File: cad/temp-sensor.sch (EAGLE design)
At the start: 68 parts, among them Q1 300S14-U, Q2 320S14-U, Q3 320S14-U, U1 SE555D, U2 SE555D, U4 MCP6001UT-I/OT, U5 MCP6001UT-I/OT, U6 MCP6001UT-I/OT, U7 MCP6001UT-I/OT, U8 NCV4264-2CST50T3G, U9 ATMEGA328P_TQFP, Y1 16MHz

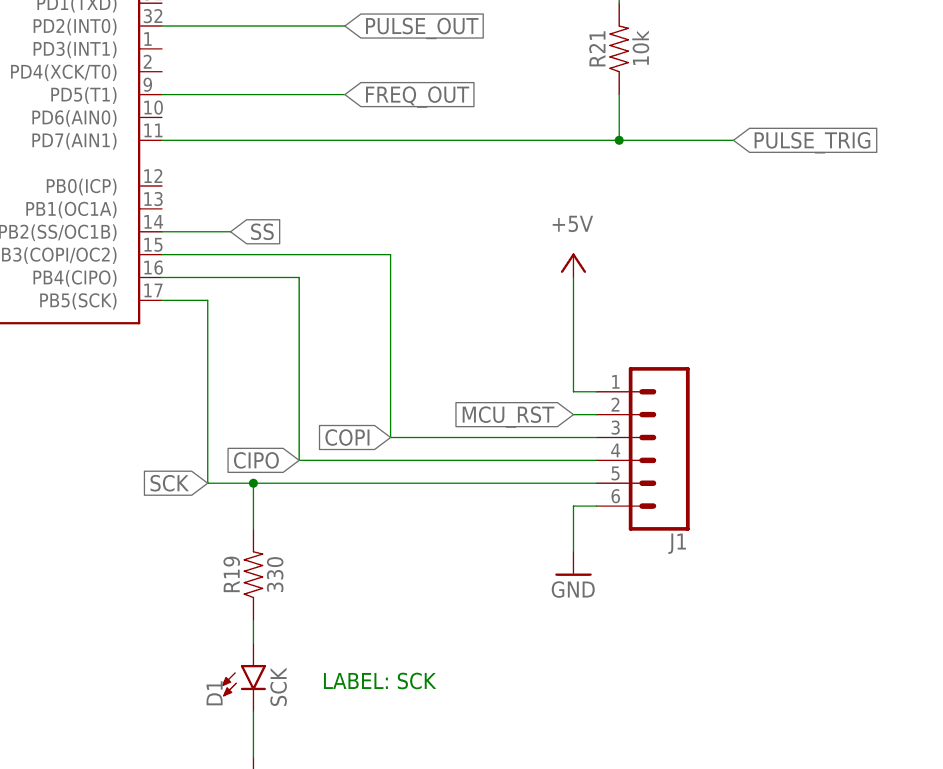
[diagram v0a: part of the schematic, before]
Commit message: Finishing touches on silk
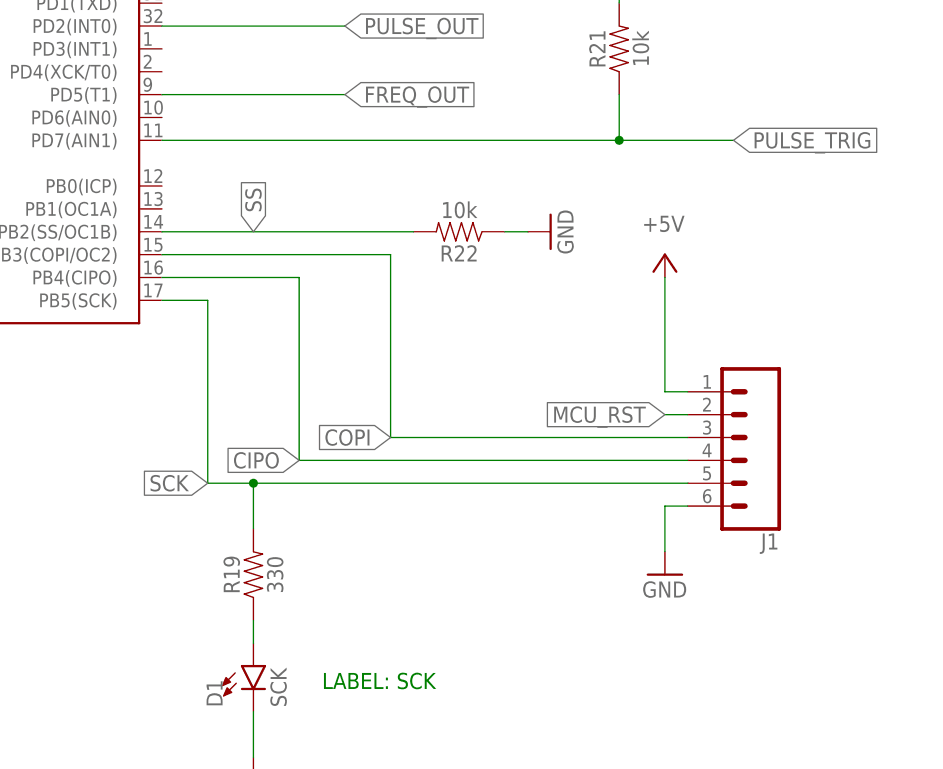
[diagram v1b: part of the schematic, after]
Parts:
- added R22: 10k, SparkFun-Resistors:10KOHM-0603-1/10W-1%
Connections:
- net GND: now also R22.1
- net SS: now also R22.2
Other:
- moved on the sheet: J1
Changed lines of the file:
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@@
 <part name="J2" library="SparkFun-Connectors" library_urn="urn:adsk.eagle:library:513" deviceset="CONN_04" device="PTH" package3d_urn="urn:adsk.eagle:package:38085/2"/>
 <part name="P+22" library="supply1" library_urn="urn:adsk.eagle:library:371" deviceset="+5V" device=""/>
+<part name="R22" library="SparkFun-Resistors" library_urn="urn:adsk.eagle:library:532" deviceset="10KOHM" device="-0603-1/10W-1%" package3d_urn="urn:adsk.eagle:package:41389018/1" value="10k"/>
+<part name="GND49" library="supply1" library_urn="urn:adsk.eagle:library:371" deviceset="GND" device=""/>
 </parts>
 <sheets>
@@
 <attribute name="VALUE" x="-177.038" y="226.06" size="1.778" layer="96" font="vector" rot="R270" align="top-center"/>
 </instance>
-<instance part="J1" gate="J1" x="-63.5" y="60.96" smashed="yes" rot="R180">
-<attribute name="VALUE" x="-58.42" y="70.866" size="1.778" layer="96" font="vector" rot="R180"/>
-<attribute name="NAME" x="-58.42" y="50.292" size="1.778" layer="95" font="vector" rot="R180"/>
-</instance>
-<instance part="GND39" gate="1" x="-71.12" y="45.72" smashed="yes">
-<attribute name="VALUE" x="-73.66" y="43.18" size="1.778" layer="96"/>
-</instance>
-<instance part="P+17" gate="1" x="-71.12" y="81.28" smashed="yes">
-<attribute name="VALUE" x="-73.66" y="83.82" size="1.778" layer="96"/>
+<instance part="J1" gate="J1" x="-53.34" y="60.96" smashed="yes" rot="R180">
+<attribute name="VALUE" x="-48.26" y="70.866" size="1.778" layer="96" font="vector" rot="R180"/>
+<attribute name="NAME" x="-48.26" y="50.292" size="1.778" layer="95" font="vector" rot="R180"/>
+</instance>
+<instance part="GND39" gate="1" x="-60.96" y="45.72" smashed="yes">
+<attribute name="VALUE" x="-63.5" y="43.18" size="1.778" layer="96"/>
+</instance>
+<instance part="P+17" gate="1" x="-60.96" y="81.28" smashed="yes">
+<attribute name="VALUE" x="-63.5" y="83.82" size="1.778" layer="96"/>
 </instance>
 <instance part="P+18" gate="1" x="-195.58" y="147.32" smashed="yes">
@@
 <instance part="P+22" gate="1" x="-38.1" y="137.16" smashed="yes">
 <attribute name="VALUE" x="-40.64" y="139.7" size="1.778" layer="96"/>
+</instance>
+<instance part="R22" gate="G$1" x="-83.82" y="83.82" smashed="yes" rot="R180">
+<attribute name="NAME" x="-83.82" y="82.296" size="1.778" layer="95" font="vector" rot="R180" align="bottom-center"/>
+<attribute name="VALUE" x="-83.82" y="85.344" size="1.778" layer="96" font="vector" rot="R180" align="top-center"/>
+</instance>
+<instance part="GND49" gate="1" x="-73.66" y="83.82" smashed="yes" rot="R90">
+<attribute name="VALUE" x="-71.12" y="81.28" size="1.778" layer="96" rot="R90"/>
 </instance>
 </instances>
@@
 <segment>
 <pinref part="J1" gate="J1" pin="6"/>
-<wire x1="-68.58" y1="53.34" x2="-71.12" y2="53.34" width="0.1524" layer="91"/>
-<wire x1="-71.12" y1="53.34" x2="-71.12" y2="48.26" width="0.1524" layer="91"/>
+<wire x1="-58.42" y1="53.34" x2="-60.96" y2="53.34" width="0.1524" layer="91"/>
+<wire x1="-60.96" y1="53.34" x2="-60.96" y2="48.26" width="0.1524" layer="91"/>
 <pinref part="GND39" gate="1" pin="GND"/>
 </segment>
@@
 <pinref part="J2" gate="J1" pin="2"/>
 <wire x1="-38.1" y1="127" x2="-35.56" y2="127" width="0.1524" layer="91"/>
+</segment>
+<segment>
+<wire x1="-78.74" y1="83.82" x2="-76.2" y2="83.82" width="0.1524" layer="91"/>
+<pinref part="GND49" gate="1" pin="GND"/>
+<pinref part="R22" gate="G$1" pin="1"/>
 </segment>
 </net>
@@
 <segment>
 <pinref part="J1" gate="J1" pin="1"/>
-<wire x1="-68.58" y1="66.04" x2="-71.12" y2="66.04" width="0.1524" layer="91"/>
-<wire x1="-71.12" y1="66.04" x2="-71.12" y2="78.74" width="0.1524" layer="91"/>
+<wire x1="-58.42" y1="66.04" x2="-60.96" y2="66.04" width="0.1524" layer="91"/>
+<wire x1="-60.96" y1="66.04" x2="-60.96" y2="78.74" width="0.1524" layer="91"/>
 <pinref part="P+17" gate="1" pin="+5V"/>
 </segment>
@@
 <segment>
 <pinref part="J1" gate="J1" pin="2"/>
-<wire x1="-68.58" y1="63.5" x2="-71.12" y2="63.5" width="0.1524" layer="91"/>
-<label x="-71.12" y="63.5" size="1.778" layer="95" rot="R180" xref="yes"/>
+<wire x1="-58.42" y1="63.5" x2="-60.96" y2="63.5" width="0.1524" layer="91"/>
+<label x="-60.96" y="63.5" size="1.778" layer="95" rot="R180" xref="yes"/>
 </segment>
 </net>
@@
 <wire x1="-111.76" y1="55.88" x2="-106.68" y2="55.88" width="0.1524" layer="91"/>
 <pinref part="R19" gate="G$1" pin="2"/>
-<wire x1="-106.68" y1="55.88" x2="-68.58" y2="55.88" width="0.1524" layer="91"/>
+<wire x1="-106.68" y1="55.88" x2="-58.42" y2="55.88" width="0.1524" layer="91"/>
 <wire x1="-106.68" y1="50.8" x2="-106.68" y2="55.88" width="0.1524" layer="91"/>
 <junction x="-106.68" y="55.88"/>
@@
 <label x="-101.6" y="58.42" size="1.778" layer="95" rot="R180" xref="yes"/>
 <pinref part="J1" gate="J1" pin="4"/>
-<wire x1="-68.58" y1="58.42" x2="-101.6" y2="58.42" width="0.1524" layer="91"/>
+<wire x1="-58.42" y1="58.42" x2="-101.6" y2="58.42" width="0.1524" layer="91"/>
 <wire x1="-101.6" y1="58.42" x2="-101.6" y2="78.74" width="0.1524" layer="91"/>
 </segment>
@@
 <pinref part="J1" gate="J1" pin="3"/>
 <wire x1="-91.44" y1="81.28" x2="-91.44" y2="60.96" width="0.1524" layer="91"/>
-<wire x1="-91.44" y1="60.96" x2="-68.58" y2="60.96" width="0.1524" layer="91"/>
+<wire x1="-91.44" y1="60.96" x2="-58.42" y2="60.96" width="0.1524" layer="91"/>
 </segment>
 </net>
@@
 <segment>
 <pinref part="U9" gate="U1" pin="PB2(SS/OC1B)"/>
-<wire x1="-116.84" y1="83.82" x2="-109.22" y2="83.82" width="0.1524" layer="91"/>
-<label x="-109.22" y="83.82" size="1.778" layer="95" xref="yes"/>
-</segment>
-</net>
+<label x="-106.68" y="83.82" size="1.778" layer="95" rot="R90" xref="yes"/>
+<pinref part="R22" gate="G$1" pin="2"/>
+<wire x1="-116.84" y1="83.82" x2="-88.9" y2="83.82" width="0.1524" layer="91"/>
+</segment>
+</net>
